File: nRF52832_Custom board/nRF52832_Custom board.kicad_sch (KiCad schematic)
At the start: 46 parts, among them J1 USB_C, J2 Battery Connector, J3 Analog, J4 PO PINS, J5 PO PINS, J6 PO PINS, J7 POWER, J8 GND, J9 Programming, SW1 SW_Push, SW2 SW_Push, U1 nRF52832-QFxx, U2 MCP73831-2-OT, U3 AP2112K-3.3, Y1 32MHZ, Y2 32.768KHZ

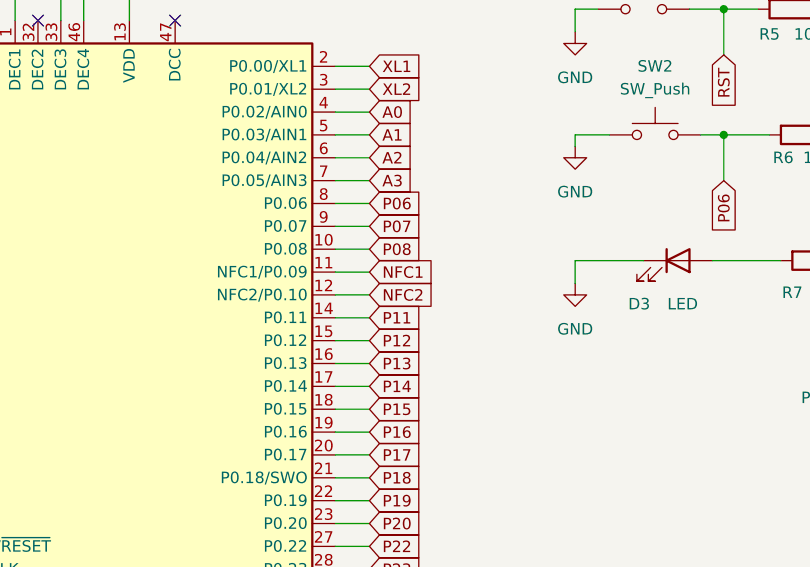
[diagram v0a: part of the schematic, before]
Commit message: updated
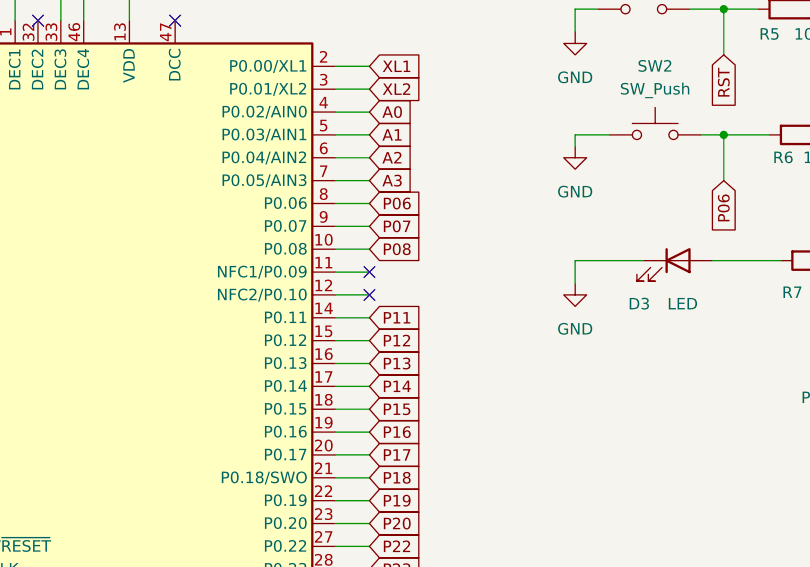
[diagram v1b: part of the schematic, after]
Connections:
- net NFC1: no longer names the net of U1.11 (NFC1/P0.09)
- net NFC2: no longer names the net of U1.12 (NFC2/P0.10)
- no-connect marks 8 -> 10
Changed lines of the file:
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@@
+	)
+	(no_connect
+		(at 275.59 59.69)
 	)
 	(no_connect
@@
 	(no_connect
 		(at 48.26 48.26)
+	)
+	(no_connect
+		(at 275.59 62.23)
 	)
 	(no_connect
@@
 		)
 	)
-	(global_label "NFC2"
-		(shape input)
-		(at 275.59 62.23 0)
+	(global_label "XC1"
+		(shape input)
+		(at 223.52 69.85 180)
+		(fields_autoplaced yes)
+		(effects
+			(font
+				(size 1.27 1.27)
+			)
+			(justify right)
+		)
+		(property "Intersheetrefs" "${INTERSHEET_REFS}"
+			(at 216.8458 69.85 0)
+			(effects
+				(font
+					(size 1.27 1.27)
+				)
+				(justify right)
+				(hide yes)
+			)
+		)
+	)
+	(global_label "P20"
+		(shape input)
+		(at 275.59 87.63 0)
 		(fields_autoplaced yes)
 		(effects
@@
 		)
 		(property "Intersheetrefs" "${INTERSHEET_REFS}"
-			(at 283.4738 62.23 0)
+			(at 282.2642 87.63 0)
 			(effects
 				(font
@@
 		)
 	)
-	(global_label "XC1"
-		(shape input)
-		(at 223.52 69.85 180)
+	(global_label "P06"
+		(shape input)
+		(at 314.96 49.53 270)
 		(fields_autoplaced yes)
 		(effects
@@
 		)
 		(property "Intersheetrefs" "${INTERSHEET_REFS}"
-			(at 216.8458 69.85 0)
+			(at 314.96 56.2042 90)
 			(effects
 				(font
@@
 		)
 	)
-	(global_label "P20"
-		(shape input)
-		(at 275.59 87.63 0)
+	(global_label "3.3V"
+		(shape input)
+		(at 389.89 110.49 0)
 		(fields_autoplaced yes)
 		(effects
@@
 		)
 		(property "Intersheetrefs" "${INTERSHEET_REFS}"
-			(at 282.2642 87.63 0)
+			(at 396.9876 110.49 0)
 			(effects
 				(font
@@
 		)
 	)
-	(global_label "P06"
-		(shape input)
-		(at 314.96 49.53 270)
-		(fields_autoplaced yes)
-		(effects
-			(font
-				(size 1.27 1.27)
-			)
-			(justify right)
-		)
-		(property "Intersheetrefs" "${INTERSHEET_REFS}"
-			(at 314.96 56.2042 90)
-			(effects
-				(font
-					(size 1.27 1.27)
-				)
-				(justify right)
+	(global_label "XL2"
+		(shape input)
+		(at 172.72 66.04 0)
+		(fields_autoplaced yes)
+		(effects
+			(font
+				(size 1.27 1.27)
+			)
+			(justify left)
+		)
+		(property "Intersheetrefs" "${INTERSHEET_REFS}"
+			(at 179.1523 66.04 0)
+			(effects
+				(font
+					(size 1.27 1.27)
+				)
+				(justify left)
+				(hide yes)
+			)
+		)
+	)
+	(global_label "P27"
+		(shape input)
+		(at 388.62 82.55 0)
+		(fields_autoplaced yes)
+		(effects
+			(font
+				(size 1.27 1.27)
+			)
+			(justify left)
+		)
+		(property "Intersheetrefs" "${INTERSHEET_REFS}"
+			(at 395.2942 82.55 0)
+			(effects
+				(font
+					(size 1.27 1.27)
+				)
+				(justify left)
+				(hide yes)
+			)
+		)
+	)
+	(global_label "STAT"
+		(shape input)
+		(at 46.99 109.22 0)
+		(fields_autoplaced yes)
+		(effects
+			(font
+				(size 1.27 1.27)
+			)
+			(justify left)
+		)
+		(property "Intersheetrefs" "${INTERSHEET_REFS}"
+			(at 54.2085 109.22 0)
+			(effects
+				(font
+					(size 1.27 1.27)
+				)
+				(justify left)
 				(hide yes)
 			)
@@
 	(global_label "3.3V"
 		(shape input)
-		(at 389.89 110.49 0)
+		(at 334.01 44.45 0)
 		(fields_autoplaced yes)
 		(effects
@@
 		)
 		(property "Intersheetrefs" "${INTERSHEET_REFS}"
-			(at 396.9876 110.49 0)
+			(at 341.1076 44.45 0)
 			(effects
 				(font
@@
 		)
 	)
-	(global_label "XL2"
-		(shape input)
-		(at 172.72 66.04 0)
+	(global_label "P24"
+		(shape input)
+		(at 361.95 93.98 0)
 		(fields_autoplaced yes)
 		(effects
@@
 		)
 		(property "Intersheetrefs" "${INTERSHEET_REFS}"
-			(at 179.1523 66.04 0)
-			(effects
-				(font
-					(size 1.27 1.27)
-				)
-				(justify left)
-				(hide yes)
-			)
-		)
-	)
-	(global_label "P27"
-		(shape input)
-		(at 388.62 82.55 0)
-		(fields_autoplaced yes)
-		(effects
-			(font
-				(size 1.27 1.27)
-			)
-			(justify left)
-		)
-		(property "Intersheetrefs" "${INTERSHEET_REFS}"
-			(at 395.2942 82.55 0)
-			(effects
-				(font
-					(size 1.27 1.27)
-				)
-				(justify left)
-				(hide yes)
-			)
-		)
-	)
-	(global_label "STAT"
-		(shape input)
-		(at 46.99 109.22 0)
-		(fields_autoplaced yes)
-		(effects
-			(font
-				(size 1.27 1.27)
-			)
-			(justify left)
-		)
-		(property "Intersheetrefs" "${INTERSHEET_REFS}"
-			(at 54.2085 109.22 0)
-			(effects
-				(font
-					(size 1.27 1.27)
-				)
-				(justify left)
-				(hide yes)
-			)
-		)
-	)
-	(global_label "3.3V"
-		(shape input)
-		(at 334.01 44.45 0)
-		(fields_autoplaced yes)
-		(effects
-			(font
-				(size 1.27 1.27)
-			)
-			(justify left)
-		)
-		(property "Intersheetrefs" "${INTERSHEET_REFS}"
-			(at 341.1076 44.45 0)
-			(effects
-				(font
-					(size 1.27 1.27)
-				)
-				(justify left)
-				(hide yes)
-			)
-		)
-	)
-	(global_label "P24"
-		(shape input)
-		(at 361.95 93.98 0)
-		(fields_autoplaced yes)
-		(effects
-			(font
-				(size 1.27 1.27)
-			)
-			(justify left)
-		)
-		(property "Intersheetrefs" "${INTERSHEET_REFS}"
 			(at 368.6242 93.98 0)
 			(effects
 				(font
-					(size 1.27 1.27)
-				)
-				(justify left)
-				(hide yes)
-			)
-		)
-	)
-	(global_label "NFC1"
-		(shape input)
-		(at 275.59 59.69 0)
-		(fields_autoplaced yes)
-		(effects
-			(font
-				(size 1.27 1.27)
-			)
-			(justify left)
-		)
-		(property "Intersheetrefs" "${INTERSHEET_REFS}"
-			(at 283.4738 59.69 0)
-			(effects
-				(font
